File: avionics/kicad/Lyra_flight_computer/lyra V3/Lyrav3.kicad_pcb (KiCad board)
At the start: 4 copper layers, 25 x 60 mm, 84 parts, among them J1 Screw_Terminal_01x08, J2 Screw_Terminal_01x06, J3 Conn_01x02, J4 Conn_01x02, J5 Conn_01x03, J6 Conn_01x06, J7 USB_B_Micro, J8 Conn_01x04, Q1 AO3401A, Q2 AO3400A, Q3 AO3400A, Q4 AO3400A, Q5 AO3400A, U1 AZ1117-3.3, U2 BMI088, U3 MPL3115A2, U4 ADXL375BCCZ-RL7, U5 LIS3MDL, U6 ADS1015IDGS, U7 W25Q64JVXGIQ, U8 RP2040, X1 S3D12.288000B20F30T

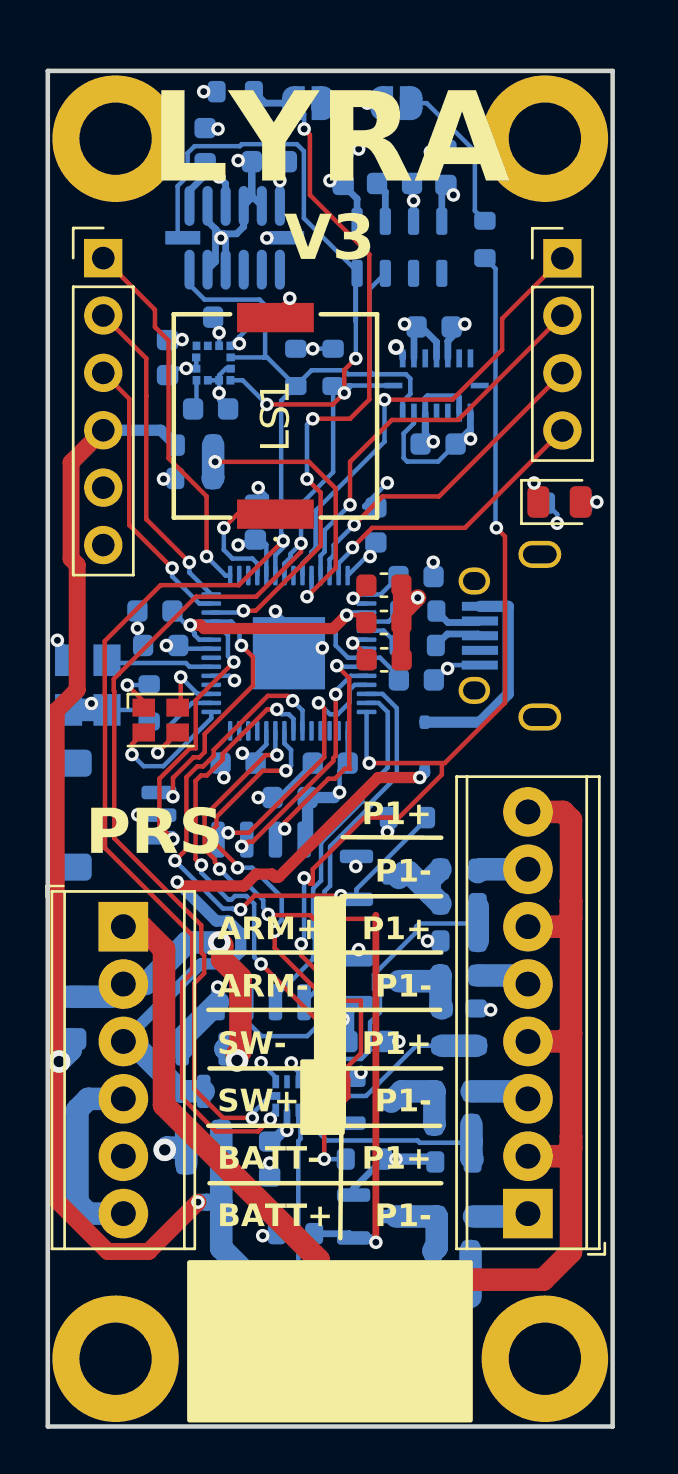
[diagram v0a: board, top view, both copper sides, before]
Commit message: more lyrav3 work
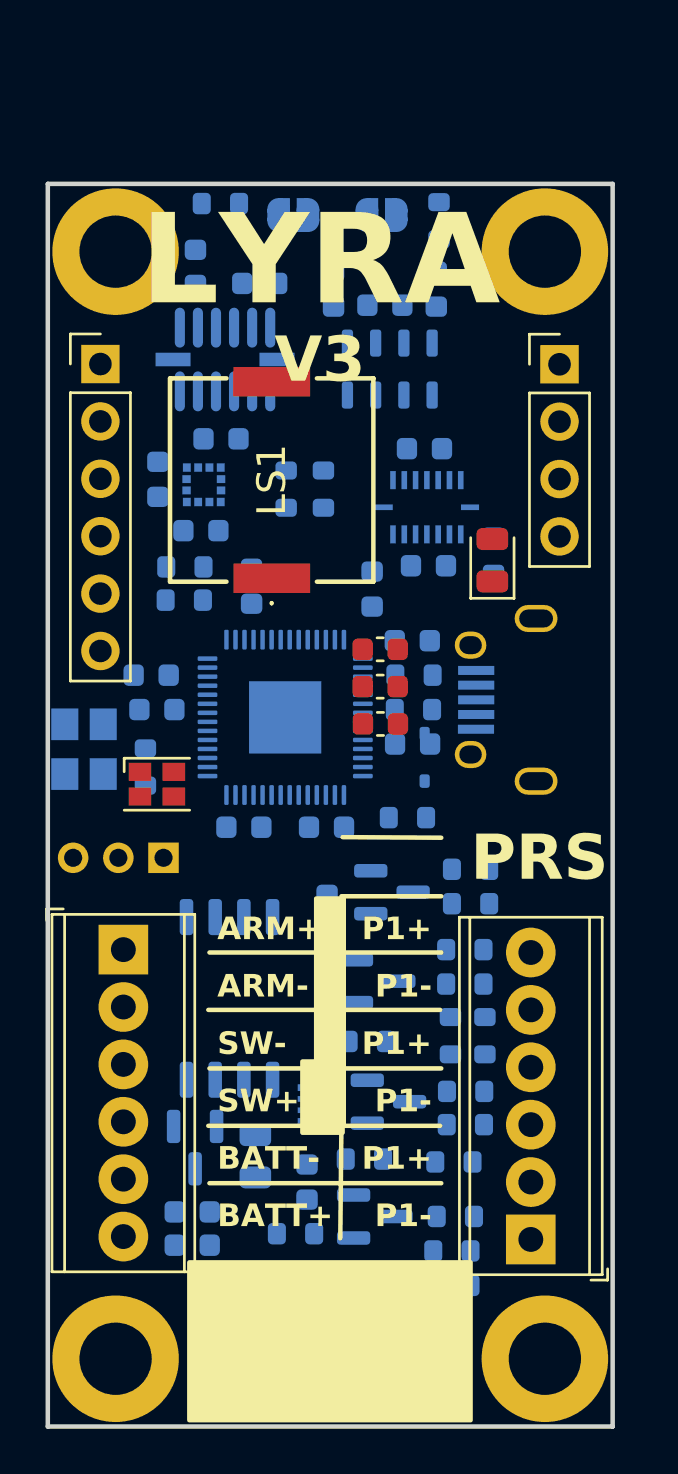
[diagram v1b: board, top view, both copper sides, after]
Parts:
- removed J1: Screw_Terminal_01x08, TerminalBlock_Phoenix:TerminalBlock_Phoenix_MPT-0,5-8-2.54_1x08_P2.54mm_Horizontal
- added J9: Screw_Terminal_01x06, TerminalBlock_Phoenix:TerminalBlock_Phoenix_MPT-0,5-6-2.54_1x06_P2.54mm_Horizontal, F.Cu at (205.0, 110.7)
- J5: footprint Connector_JST:JST_SH_SM03B-SRSS-TB_1x03-1MP_P1.00mm_Horizontal -> Connector_PinHeader_2.00mm:PinHeader_1x03_P2.00mm_Vertical
- moved F1 10.2 mm to (192.8, 107.1)
- moved C3 5.40 mm to (196.2, 68.7)
- moved C4 5.40 mm to (200.8, 68.7)
- moved C1 5.40 mm to (200.4, 80.9)
- moved C10 5.40 mm to (193.0, 68.4)
- moved C12 5.40 mm to (188.5, 77.1)
- moved C13 5.40 mm to (191.3, 75.3)
- moved C14 5.40 mm to (190.4, 79.4)
- moved C2 5.40 mm to (200.3, 75.7)
- moved C9 5.40 mm to (198.5, 69.4)
- moved R4 5.40 mm to (189.7, 81.0)
- moved R5 5.40 mm to (189.6, 82.4)
- moved R6 5.40 mm to (195.8, 77.5)
- moved R7 5.40 mm to (194.1, 77.5)
- moved U2 5.40 mm to (200.4, 78.3)
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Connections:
- J2 pad 1: /PYRO PWR -> /P4-
- J2 pad 2: +12P -> /PYRO PWR
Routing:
- net /I2C1 SCL: track 77.1 -> 0.00 mm, vias 5 -> 0
- net GND: track 76.6 -> 0.00 mm, vias 44 -> 0
- net /I2C1 SDA: track 68.2 -> 0.00 mm, vias 2 -> 0
- net +12VA: track 66.1 -> 0.00 mm, vias 2 -> 0
- net /PYRO PWR: track 62.2 -> 0.00 mm
- net +3V3: track 58.4 -> 0.00 mm, vias 24 -> 0
- net /QSPI_SS: track 44.8 -> 0.00 mm, vias 5 -> 0
- net /P4 EN : track 33.6 -> 0.00 mm, vias 4 -> 0
- net /RUN: track 31.4 -> 0.00 mm, vias 4 -> 0
- net +12V: track 29.4 -> 0.00 mm, vias 2 -> 0
- net /P3 EN : track 28.0 -> 0.00 mm, vias 5 -> 0
- net /P1 EN : track 25.2 -> 0.00 mm, vias 4 -> 0
- net /P2 EN : track 24.2 -> 0.00 mm, vias 4 -> 0
- net /QSPI_SD2: track 22.3 -> 0.00 mm
- net /BRKOUT1: track 20.6 -> 0.00 mm, vias 1 -> 0
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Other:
- board size 25 x 60 mm -> 25 x 55 mm
